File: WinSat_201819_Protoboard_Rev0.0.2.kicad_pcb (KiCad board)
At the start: 4 copper layers, 46.7 x 59.5 mm, 74 parts, among them J1 Conn_01x02_Female, J10 Conn_01x06_Male, J11 USB_B_Micro, J2 Conn_01x02_Female, J3 Conn_01x02_Female, J4 Conn_01x02_Female, J5 Conn_01x03_Female, J6 Conn_01x02_Female, J7 JTAG-6PIN, J8 Conn_01x03_Female, J9 Conn_01x03_Female, P1 TPS82150, Q1 SSM3K329R, Q2 SSM3K329R, Q3 SSM3K329R, Q4 Package_TO_SOT_SMD:SOT-23, U1 LTC4361, U10 XBEE_PRO900, U2 Si1470DH, U3 BMP280, U9 ATxmega128A4-AU

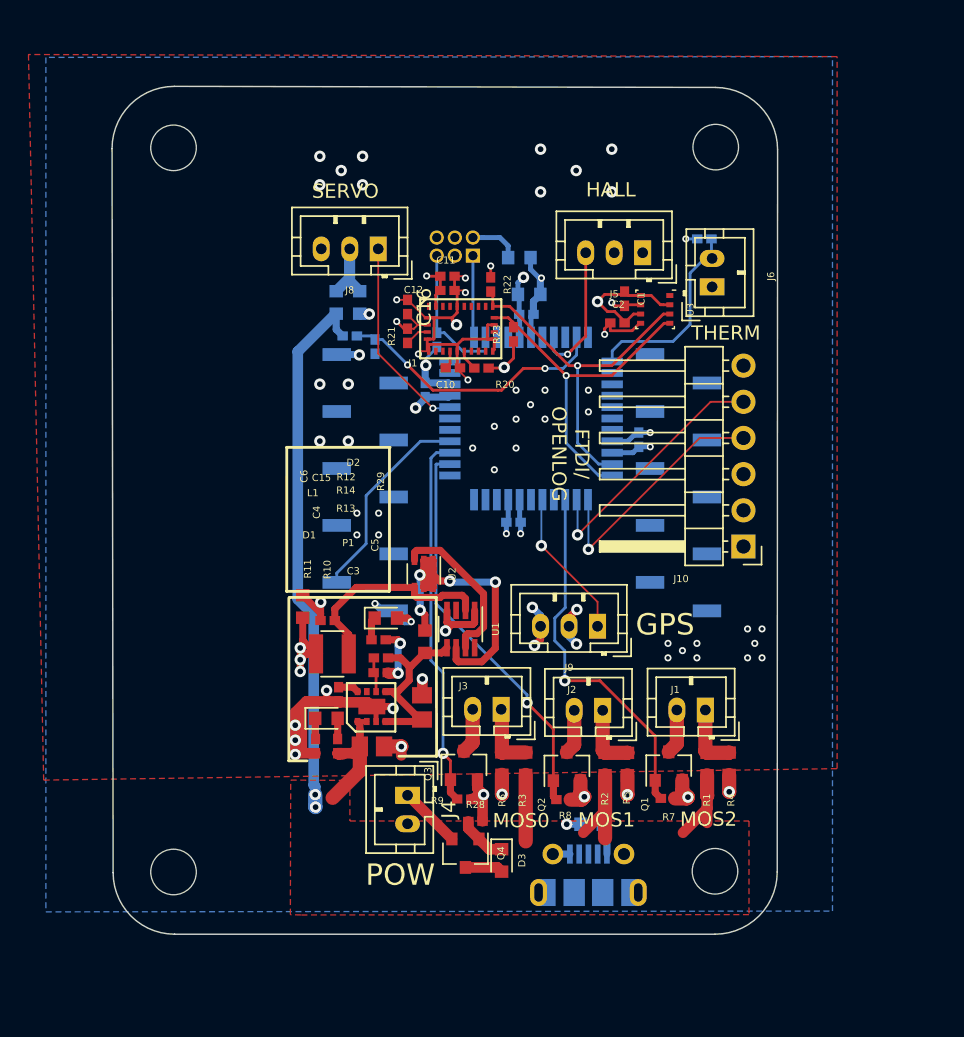
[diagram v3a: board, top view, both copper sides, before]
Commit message: Make sure updated
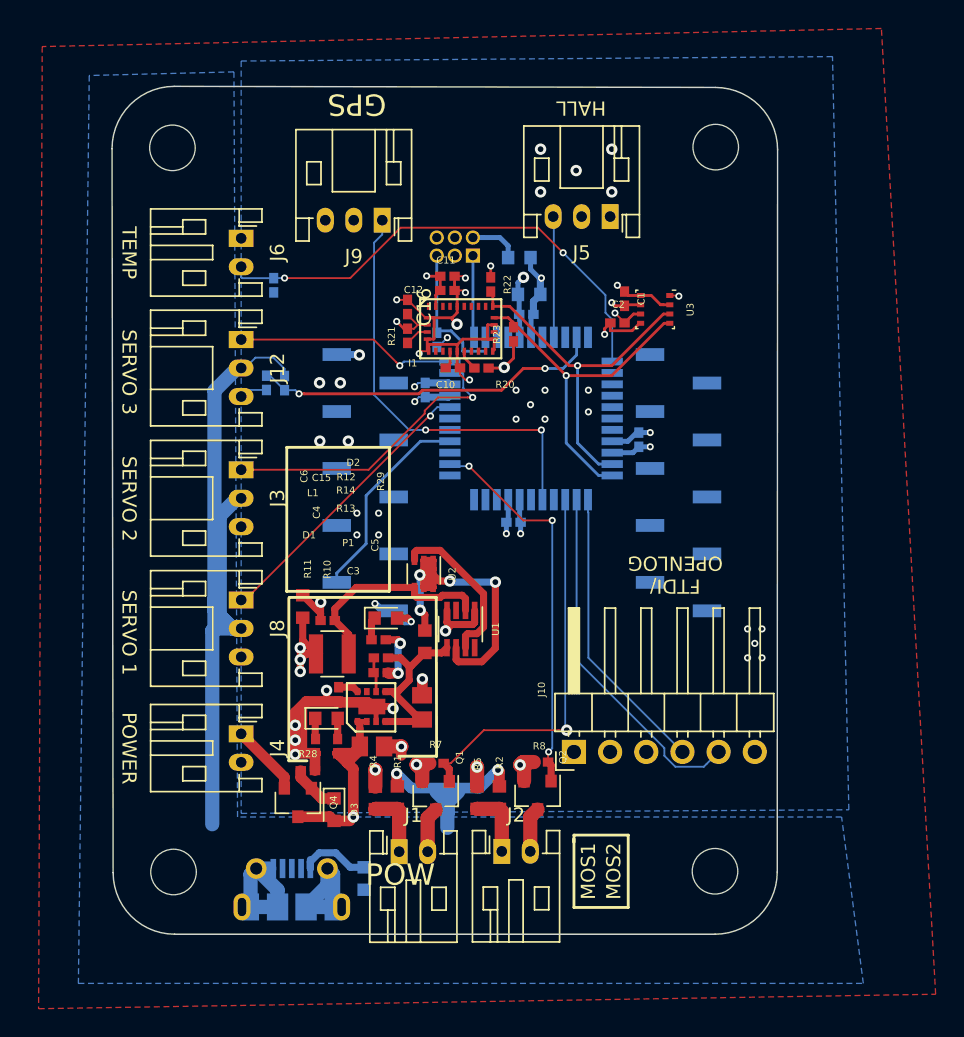
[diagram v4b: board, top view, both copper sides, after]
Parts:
- removed Q3: SSM3K329R, Package_TO_SOT_SMD:SOT-23
- removed R15, R16: R_Small, Resistor_SMD:R_0603_1608Metric
- removed R3, R6: 0 OHM, Resistor_SMD:R_0603_1608Metric
- removed R9: 100K, OSD335x-KiCad-master:Not_Broken_0402
- added J12: Conn_01x03_Female, Connector_JST:JST_PH_S3B-PH-K_1x03_P2.00mm_Horizontal, F.Cu at (62.0, 86.9)
- J1, J2, J4, J6: footprint Connector_JST:JST_PH_B2B-PH-K_1x02_P2.00mm_Vertical -> Connector_JST:JST_PH_S2B-PH-K_1x02_P2.00mm_Horizontal
- J3: value Conn_01x02_Female -> Conn_01x03_Female; footprint Connector_JST:JST_PH_B2B-PH-K_1x02_P2.00mm_Vertical -> Connector_JST:JST_PH_S3B-PH-K_1x03_P2.00mm_Horizontal
- J5, J8, J9: footprint Connector_JST:JST_PH_B3B-PH-K_1x03_P2.00mm_Vertical -> Connector_JST:JST_PH_S3B-PH-K_1x03_P2.00mm_Horizontal
- moved J6 33.2 mm to (62.0, 79.8), turned to 270 degrees
- moved J9 32.3 mm to (71.9, 78.5)
- moved R26 30.4 mm to (64.3, 83.1), turned to 90 degrees
- moved J8 26.5 mm to (62.0, 105.2), turned to 270 degrees
- moved R4 25.0 mm to (71.4, 119.1), turned to 90 degrees
- moved J3 24.8 mm to (62.0, 96.0), turned to 270 degrees
- moved J1 23.7 mm to (73.1, 122.8), turned to 0 degrees
- moved R1 21.9 mm to (72.9, 119.0), turned to 90 degrees
- moved J11 20.9 mm to (65.5, 125.5)
- moved J10 18.7 mm to (85.3, 115.8), turned to 90 degrees
- moved Q1 16.5 mm to (75.6, 118.9), turned to 270 degrees
- moved R7 16.4 mm to (75.7, 116.6), turned to 180 degrees
- moved D4 16.4 mm to (70.6, 124.7), turned to 270 degrees
- moved J4 12.5 mm to (62.0, 114.6)
- moved Q4 12.3 mm to (66.0, 119.4)
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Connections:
- net SERVO_TCL renamed SERVO_TCL_1
- J3 pad 1: Net-(J3-Pad1) -> SERVO_TCL_2
- J3 pad 2: Net-(J3-Pad2) -> BAT_POS
- J8 pad 2: Net-(J8-Pad2) -> BAT_POS
- U9 pad 32: Net-(U9-Pad32) -> SERVO_TCL_2
- U9 pad 33: Net-(U9-Pad33) -> SERVO_TCL_3
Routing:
- net MOSFET2_GPIO: track 26.2 -> 0.00 mm, vias 1 -> 0
- net SERVO_TCL_2: track 0.00 -> 21.4 mm, vias 0 -> 1
- net TEMP_SENSE-ADC: track 14.0 -> 34.7 mm, vias 0 -> 2
- net GPS_TX-MCU_RX: track 10.6 -> 30.3 mm, vias 1 -> 2
- net SERVO_TCL_3: track 0.00 -> 15.5 mm, vias 0 -> 1
- net GND: track 99.6 -> 111.8 mm, vias 69 -> 49
- net +3V3: track 53.6 -> 44.3 mm, vias 19 -> 18
- net FTDI_OLOG_RX-MCU_TX: track 18.0 -> 25.2 mm, vias 1 -> 0
- net Net-(J8-Pad2): track 6.63 -> 0.00 mm
- net SERVO_TCL_1: track 14.0 -> 20.5 mm
- net BAT_POS: track 78.8 -> 84.5 mm
- net VOLTDIV_ADC: track 19.3 -> 24.7 mm
- net Net-(J3-Pad1): track 4.72 -> 0.00 mm
- net Net-(D4-Pad1): track 2.21 -> 5.56 mm
- net Net-(J3-Pad2): track 3.19 -> 0.00 mm
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- added copper zone on B.Cu, net BAT_POS
- removed copper zone on F.Cu, net BAT_POS
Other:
- board text added: "POWER"
- board text added: "SERVO 1"
- board text added: "SERVO 2"
- board text added: "SERVO 3"
- board text added: "TEMP"
- board text removed: "MOS0"
- board text removed: "SERVO"
- board text removed: "THERM"
